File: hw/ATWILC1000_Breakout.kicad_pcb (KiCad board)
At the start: 2 copper layers, 34.9 x 38 mm, 16 parts, among them IC1 ATWILC1000-MR110PB-T, J1 Conn_02x03_Odd_Even, J2 I2C_Conn_01x03, J3 Misc_Conn_02x03, J4 GPIO_Conn_01x04, J5 UART_Conn_01x03, J6 SPI_Conn_02x04

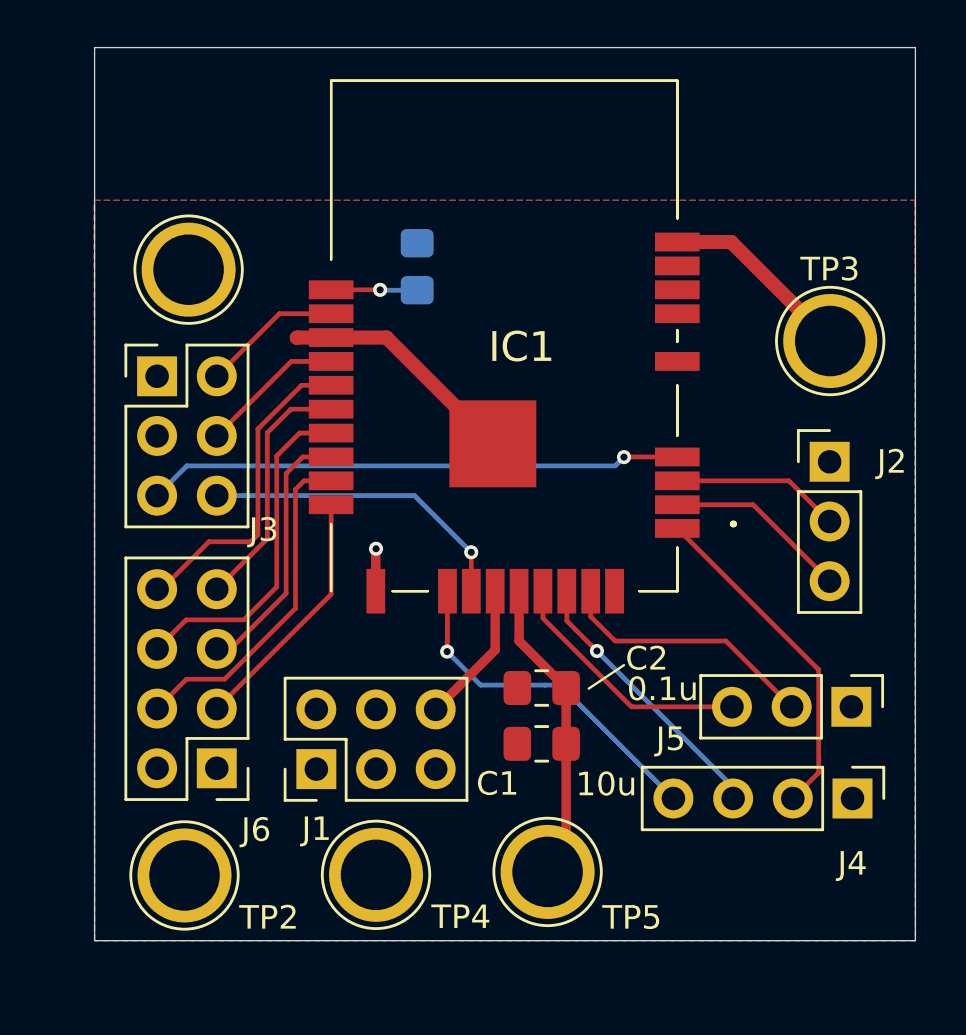
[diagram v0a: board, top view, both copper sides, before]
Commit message: finished and ordered board
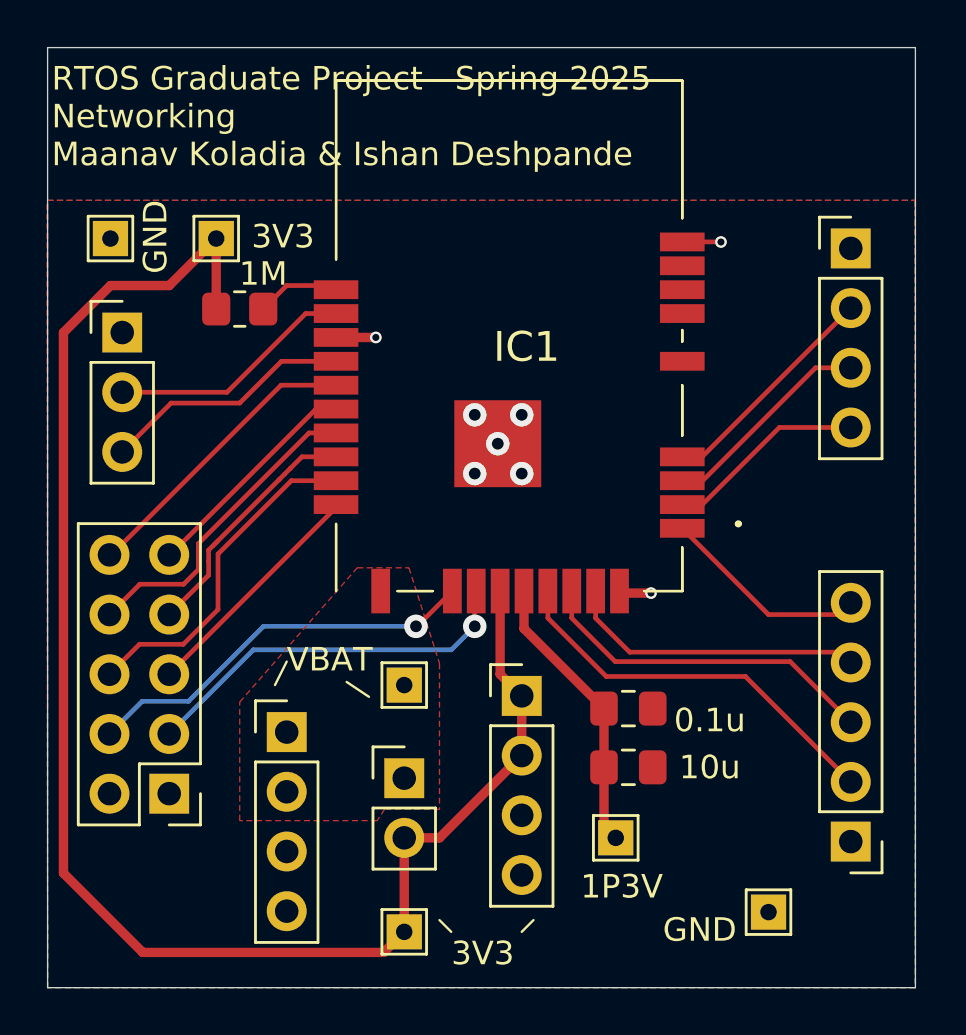
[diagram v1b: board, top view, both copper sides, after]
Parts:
- removed the G*** at (149.5, 99.6)
- removed the J4 at (161.6, 115.8)
- added G***: LOGO, hw:troll, B.Cu at (148.7, 98.9)
- added J2: VBAT_Conn_01x04, Connector_PinHeader_2.54mm:PinHeader_1x04_P2.54mm_Vertical, F.Cu at (137.5, 113.0)
- added J5: VBAT_3V3_Jump_Conn_01x02, Connector_PinHeader_2.54mm:PinHeader_1x02_P2.54mm_Vertical, F.Cu at (142.5, 115.0)
- added TP3: VBAT, TestPoint:TestPoint_THTPad_1.5x1.5mm_Drill0.7mm, F.Cu at (142.5, 111.0)
- J1: value Conn_02x03_Odd_Even -> 3V3_Conn_01x04; footprint Connector_PinHeader_2.54mm:PinHeader_2x03_P2.54mm_Vertical -> Connector_PinHeader_2.54mm:PinHeader_1x04_P2.54mm_Vertical
- J3: renamed from J2; value I2C_Conn_01x03 -> I2C_CEN_Conn_01x04; footprint Connector_PinHeader_2.54mm:PinHeader_1x03_P2.54mm_Vertical -> Connector_PinHeader_2.54mm:PinHeader_1x04_P2.54mm_Vertical
- J4: renamed from J3; value Misc_Conn_02x03 -> Misc_Conn_01x03; footprint Connector_PinHeader_2.54mm:PinHeader_2x03_P2.54mm_Vertical -> Connector_PinHeader_2.54mm:PinHeader_1x03_P2.54mm_Vertical
- J6: renamed from J5; value UART_Conn_01x03 -> UART_Conn_01x05; footprint Connector_PinHeader_2.54mm:PinHeader_1x03_P2.54mm_Vertical -> Connector_PinHeader_2.54mm:PinHeader_1x05_P2.54mm_Vertical
- J7: renamed from J6; value SPI_Conn_02x04 -> SPI_Conn_02x05; footprint Connector_PinHeader_2.54mm:PinHeader_2x04_P2.54mm_Vertical -> Connector_PinHeader_2.54mm:PinHeader_2x05_P2.54mm_Vertical
- R1: moved to F.Cu
- TP1: footprint TestPoint:TestPoint_Plated_Hole_D3.0mm -> TestPoint:TestPoint_THTPad_1.5x1.5mm_Drill0.7mm
- TP2: renamed from TP4; footprint TestPoint:TestPoint_Plated_Hole_D3.0mm -> TestPoint:TestPoint_THTPad_1.5x1.5mm_Drill0.7mm
- TP4: renamed from TP2; footprint TestPoint:TestPoint_Plated_Hole_D3.0mm -> TestPoint:TestPoint_THTPad_1.5x1.5mm_Drill0.7mm
- TP5: renamed from TP3; footprint TestPoint:TestPoint_Plated_Hole_D3.0mm -> TestPoint:TestPoint_THTPad_1.5x1.5mm_Drill0.7mm
- TP7: renamed from TP5; footprint TestPoint:TestPoint_Plated_Hole_D3.0mm -> TestPoint:TestPoint_THTPad_1.5x1.5mm_Drill0.7mm
- moved TP5 30.9 mm to (130.0, 92.0)
- moved TP2 16.8 mm to (158.0, 120.7), turned to 180 degrees
- moved TP4 9.65 mm to (142.5, 121.5)
- moved J1 9.28 mm to (147.5, 111.5), turned to 0 degrees
- moved J3 9.12 mm to (161.5, 92.4)
- moved R1 7.76 mm to (135.5, 95.0), turned to 0 degrees
- moved J6 5.74 mm to (161.5, 117.7), turned to 180 degrees
- moved C1 3.82 mm to (152.0, 114.5), turned to 0 degrees
- moved C2 3.79 mm to (152.0, 112.0), turned to 0 degrees
- moved TP7 3.24 mm to (151.5, 117.5)
- moved J4 2.38 mm to (130.5, 96.0)
- moved J7 2.30 mm to (132.5, 115.6)
- moved TP1 1.77 mm to (134.5, 92.0)
- moved IC1 0.21 mm to (147.0, 96.1)
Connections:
- IC1 pad J20: +3.3V -> /VBAT
- J1 pad 1: GND -> +3.3V
- J1 pad 4: +3.3V -> GND
- J3 pad 2: /I2C_SDA -> /RESET_N
- J3 pad 3: /I2C_SCL -> /I2C_SDA
- J4 pad 3: unconnected-(J3-Pin_3-Pad3) -> /IRQN
- J6 pad 2: /UART_TX -> /UART_RX
- J6 pad 3: /UART_RX -> /GPIO_4
- J7 pad 3: /SD_CLK -> /C_EN
- J7 pad 4: /SPI_CLK -> /GPIO_1
- J7 pad 5: /SPI_SDO -> /SD_CLK
- J7 pad 6: /SPI_CS -> /SPI_CLK
- J7 pad 7: /SPI_SDI -> /SPI_SDO
- J7 pad 8: /SD_DAT3 -> /SPI_CS
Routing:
- net +3.3V: track 7.90 -> 68.2 mm, vias 1 -> 0
- net GND: track 18.5 -> 4.72 mm, vias 0 -> 8
- net /RESET_N: track 22.8 -> 9.79 mm, vias 1 -> 0
- net /UART_RX: track 10.8 -> 16.9 mm
- net /GPIO_6: track 14.4 -> 8.90 mm
- net /IRQN: track 6.18 -> 10.7 mm
- net /WAKE: track 5.97 -> 10.5 mm
- net /GPIO_4: track 11.8 -> 14.9 mm, vias 1 -> 0
- net /C_EN: track 13.5 -> 16.4 mm
- net /GPIO_1: track 14.8 -> 17.1 mm
- net /I2C_SDA: track 7.20 -> 9.16 mm
- net /UART_TX: track 11.2 -> 12.8 mm
- net /SPI_SDI: track 10.7 -> 9.67 mm
- net /SD_DAT3: track 13.6 -> 12.6 mm
- net /SPI_CS: track 14.5 -> 13.5 mm
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- added copper zone on F.Cu, net /VBAT
- added copper zone on B.Cu, net GND
- removed copper zone on B.Cu, net +3.3V
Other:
- board size 34.9 x 38 mm -> 36.9 x 40 mm
- board text added: "1P3V"
- board text added: "3V3"
- board text added: "GND"
- board text added: "RTOS Graduate Project - Spring 2025 Networking Maanav Koladia & Ishan Deshpande"
- board text added: "VBAT"
- board text removed: "RTOS Graduate Project Networking Maanav Koladia & Ishan Deshpande"
